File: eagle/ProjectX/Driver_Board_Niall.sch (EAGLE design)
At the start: 25 parts, among them IC2 NCV78M05BDTRKG, J1 694102303002, Q2 2N7002, U1 CD74HC4067SM96, U2 ADA4091-2ARZ-RL, U35 TC4427AEOA, X1 1296-T50, X2 1296-T50

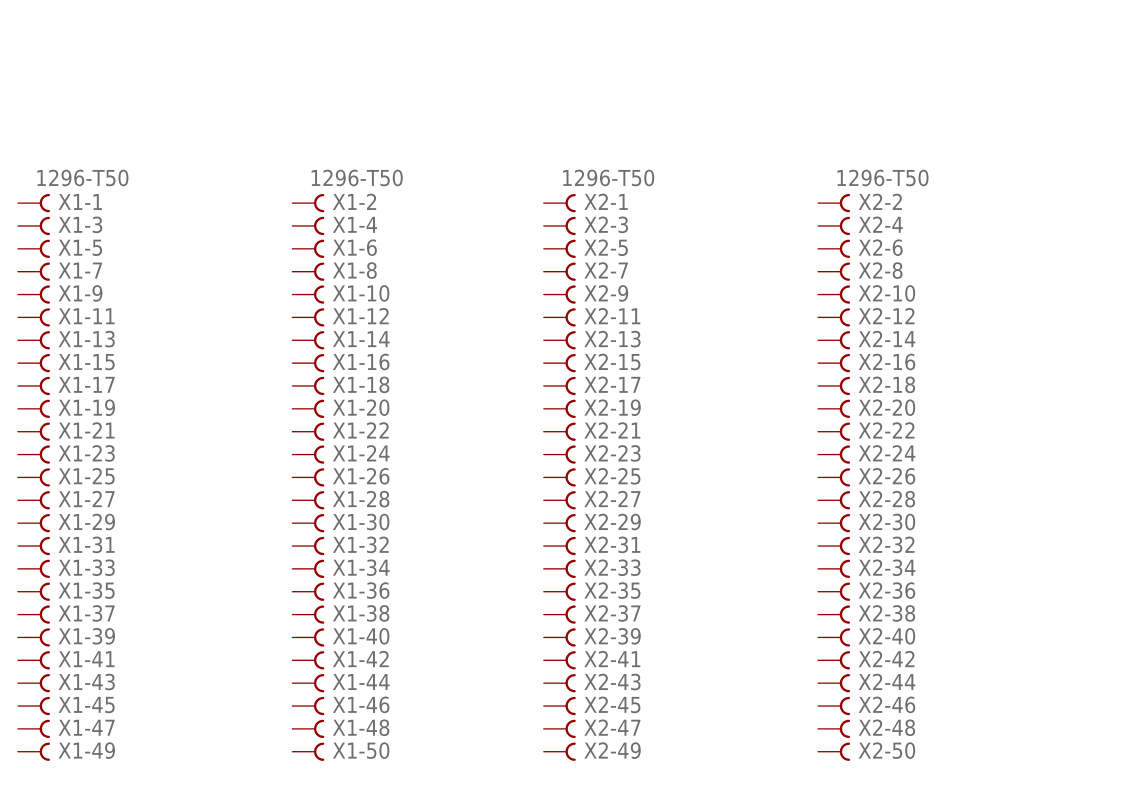
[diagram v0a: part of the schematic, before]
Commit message: Niall board edits
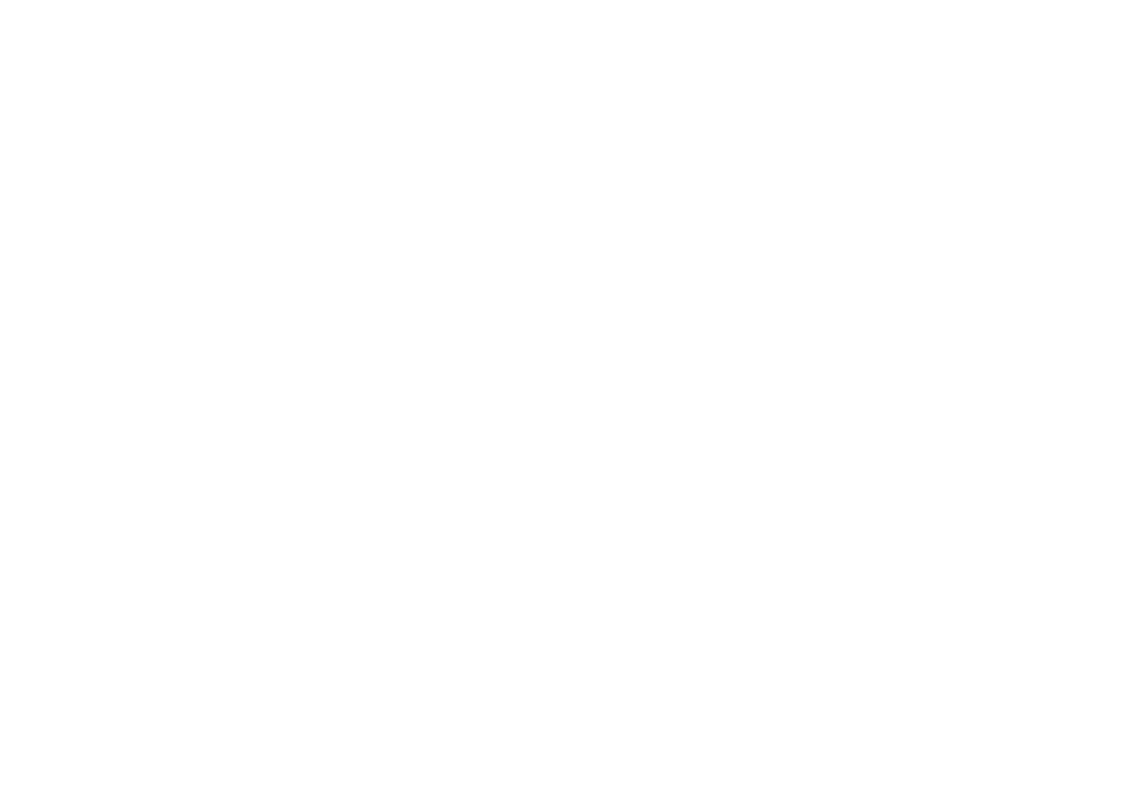
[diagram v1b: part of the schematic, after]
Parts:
- removed X1, X2: 1296-T50, con-leotronics:1296-T50
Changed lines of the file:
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@@
 <part name="U1" library="SnapEDA-Library (3)" deviceset="CD74HC4067SM96" device=""/>
 <part name="SUPPLY2" library="supply1" library_urn="urn:adsk.eagle:library:371" deviceset="GND" device=""/>
-<part name="X1" library="con-leotronics" library_urn="urn:adsk.eagle:library:160" deviceset="1296-T50" device="" package3d_urn="urn:adsk.eagle:package:7940/1"/>
-<part name="X2" library="con-leotronics" library_urn="urn:adsk.eagle:library:160" deviceset="1296-T50" device="" package3d_urn="urn:adsk.eagle:package:7940/1"/>
 </parts>
 <sheets>
@@
 <instance part="U1" gate="A" x="213.36" y="233.68"/>
 <instance part="SUPPLY2" gate="1" x="187.96" y="190.5" rot="MR0"/>
-<instance part="X1" gate="-1" x="-287.02" y="38.1"/>
-<instance part="X1" gate="-2" x="-256.54" y="38.1"/>
-<instance part="X1" gate="-3" x="-287.02" y="35.56"/>
-<instance part="X1" gate="-4" x="-256.54" y="35.56"/>
-<instance part="X1" gate="-5" x="-287.02" y="33.02"/>
-<instance part="X1" gate="-6" x="-256.54" y="33.02"/>
-<instance part="X1" gate="-7" x="-287.02" y="30.48"/>
-<instance part="X1" gate="-8" x="-256.54" y="30.48"/>
-<instance part="X1" gate="-9" x="-287.02" y="27.94"/>
-<instance part="X1" gate="-10" x="-256.54" y="27.94"/>
-<instance part="X1" gate="-11" x="-287.02" y="25.4"/>
-<instance part="X1" gate="-12" x="-256.54" y="25.4"/>
-<instance part="X1" gate="-13" x="-287.02" y="22.86"/>
-<instance part="X1" gate="-14" x="-256.54" y="22.86"/>
-<instance part="X1" gate="-15" x="-287.02" y="20.32"/>
-<instance part="X1" gate="-16" x="-256.54" y="20.32"/>
-<instance part="X1" gate="-17" x="-287.02" y="17.78"/>
-<instance part="X1" gate="-18" x="-256.54" y="17.78"/>
-<instance part="X1" gate="-19" x="-287.02" y="15.24"/>
-<instance part="X1" gate="-20" x="-256.54" y="15.24"/>
-<instance part="X1" gate="-21" x="-287.02" y="12.7"/>
-<instance part="X1" gate="-22" x="-256.54" y="12.7"/>
-<instance part="X1" gate="-23" x="-287.02" y="10.16"/>
-<instance part="X1" gate="-24" x="-256.54" y="10.16"/>
-<instance part="X1" gate="-25" x="-287.02" y="7.62"/>
-<instance part="X1" gate="-26" x="-256.54" y="7.62"/>
-<instance part="X1" gate="-27" x="-287.02" y="5.08"/>
-<instance part="X1" gate="-28" x="-256.54" y="5.08"/>
-<instance part="X1" gate="-29" x="-287.02" y="2.54"/>
-<instance part="X1" gate="-30" x="-256.54" y="2.54"/>
-<instance part="X1" gate="-31" x="-287.02" y="0"/>
-<instance part="X1" gate="-32" x="-256.54" y="0"/>
-<instance part="X1" gate="-33" x="-287.02" y="-2.54"/>
-<instance part="X1" gate="-34" x="-256.54" y="-2.54"/>
-<instance part="X1" gate="-35" x="-287.02" y="-5.08"/>
-<instance part="X1" gate="-36" x="-256.54" y="-5.08"/>
-<instance part="X1" gate="-37" x="-287.02" y="-7.62"/>
-<instance part="X1" gate="-38" x="-256.54" y="-7.62"/>
-<instance part="X1" gate="-39" x="-287.02" y="-10.16"/>
-<instance part="X1" gate="-40" x="-256.54" y="-10.16"/>
-<instance part="X1" gate="-41" x="-287.02" y="-12.7"/>
-<instance part="X1" gate="-42" x="-256.54" y="-12.7"/>
-<instance part="X1" gate="-43" x="-287.02" y="-15.24"/>
-<instance part="X1" gate="-44" x="-256.54" y="-15.24"/>
-<instance part="X1" gate="-45" x="-287.02" y="-17.78"/>
-<instance part="X1" gate="-46" x="-256.54" y="-17.78"/>
-<instance part="X1" gate="-47" x="-287.02" y="-20.32"/>
-<instance part="X1" gate="-48" x="-256.54" y="-20.32"/>
-<instance part="X1" gate="-49" x="-287.02" y="-22.86"/>
-<instance part="X1" gate="-50" x="-256.54" y="-22.86"/>
-<instance part="X2" gate="-1" x="-228.6" y="38.1"/>
-<instance part="X2" gate="-2" x="-198.12" y="38.1"/>
-<instance part="X2" gate="-3" x="-228.6" y="35.56"/>
-<instance part="X2" gate="-4" x="-198.12" y="35.56"/>
-<instance part="X2" gate="-5" x="-228.6" y="33.02"/>
-<instance part="X2" gate="-6" x="-198.12" y="33.02"/>
-<instance part="X2" gate="-7" x="-228.6" y="30.48"/>
-<instance part="X2" gate="-8" x="-198.12" y="30.48"/>
-<instance part="X2" gate="-9" x="-228.6" y="27.94"/>
-<instance part="X2" gate="-10" x="-198.12" y="27.94"/>
-<instance part="X2" gate="-11" x="-228.6" y="25.4"/>
-<instance part="X2" gate="-12" x="-198.12" y="25.4"/>
-<instance part="X2" gate="-13" x="-228.6" y="22.86"/>
-<instance part="X2" gate="-14" x="-198.12" y="22.86"/>
-<instance part="X2" gate="-15" x="-228.6" y="20.32"/>
-<instance part="X2" gate="-16" x="-198.12" y="20.32"/>
-<instance part="X2" gate="-17" x="-228.6" y="17.78"/>
-<instance part="X2" gate="-18" x="-198.12" y="17.78"/>
-<instance part="X2" gate="-19" x="-228.6" y="15.24"/>
-<instance part="X2" gate="-20" x="-198.12" y="15.24"/>
-<instance part="X2" gate="-21" x="-228.6" y="12.7"/>
-<instance part="X2" gate="-22" x="-198.12" y="12.7"/>
-<instance part="X2" gate="-23" x="-228.6" y="10.16"/>
-<instance part="X2" gate="-24" x="-198.12" y="10.16"/>
-<instance part="X2" gate="-25" x="-228.6" y="7.62"/>
-<instance part="X2" gate="-26" x="-198.12" y="7.62"/>
-<instance part="X2" gate="-27" x="-228.6" y="5.08"/>
-<instance part="X2" gate="-28" x="-198.12" y="5.08"/>
-<instance part="X2" gate="-29" x="-228.6" y="2.54"/>
-<instance part="X2" gate="-30" x="-198.12" y="2.54"/>
-<instance part="X2" gate="-31" x="-228.6" y="0"/>
-<instance part="X2" gate="-32" x="-198.12" y="0"/>
-<instance part="X2" gate="-33" x="-228.6" y="-2.54"/>
-<instance part="X2" gate="-34" x="-198.12" y="-2.54"/>
-<instance part="X2" gate="-35" x="-228.6" y="-5.08"/>
-<instance part="X2" gate="-36" x="-198.12" y="-5.08"/>
-<instance part="X2" gate="-37" x="-228.6" y="-7.62"/>
-<instance part="X2" gate="-38" x="-198.12" y="-7.62"/>
-<instance part="X2" gate="-39" x="-228.6" y="-10.16"/>
-<instance part="X2" gate="-40" x="-198.12" y="-10.16"/>
-<instance part="X2" gate="-41" x="-228.6" y="-12.7"/>
-<instance part="X2" gate="-42" x="-198.12" y="-12.7"/>
-<instance part="X2" gate="-43" x="-228.6" y="-15.24"/>
-<instance part="X2" gate="-44" x="-198.12" y="-15.24"/>
-<instance part="X2" gate="-45" x="-228.6" y="-17.78"/>
-<instance part="X2" gate="-46" x="-198.12" y="-17.78"/>
-<instance part="X2" gate="-47" x="-228.6" y="-20.32"/>
-<instance part="X2" gate="-48" x="-198.12" y="-20.32"/>
-<instance part="X2" gate="-49" x="-228.6" y="-22.86"/>
-<instance part="X2" gate="-50" x="-198.12" y="-22.86"/>
 </instances>
 <busses>
